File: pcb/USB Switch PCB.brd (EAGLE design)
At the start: 26.7 x 77.5 mm, 28 parts, among them Q1 2N7002P, Q2 2N7002P, U1 D1MINI, X1 AMPHENOL-0001LF, X2 UE27-USBA

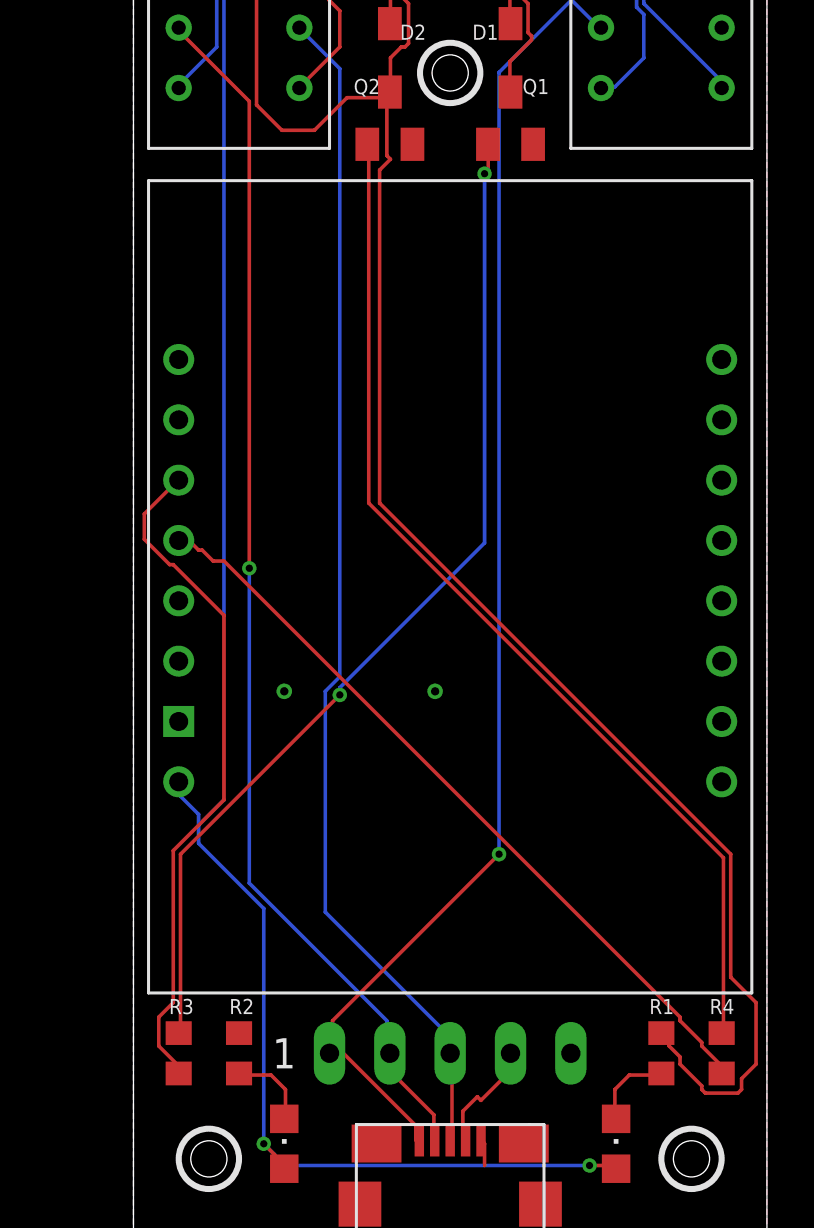
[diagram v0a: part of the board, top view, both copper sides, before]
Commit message: Working on new board revision.
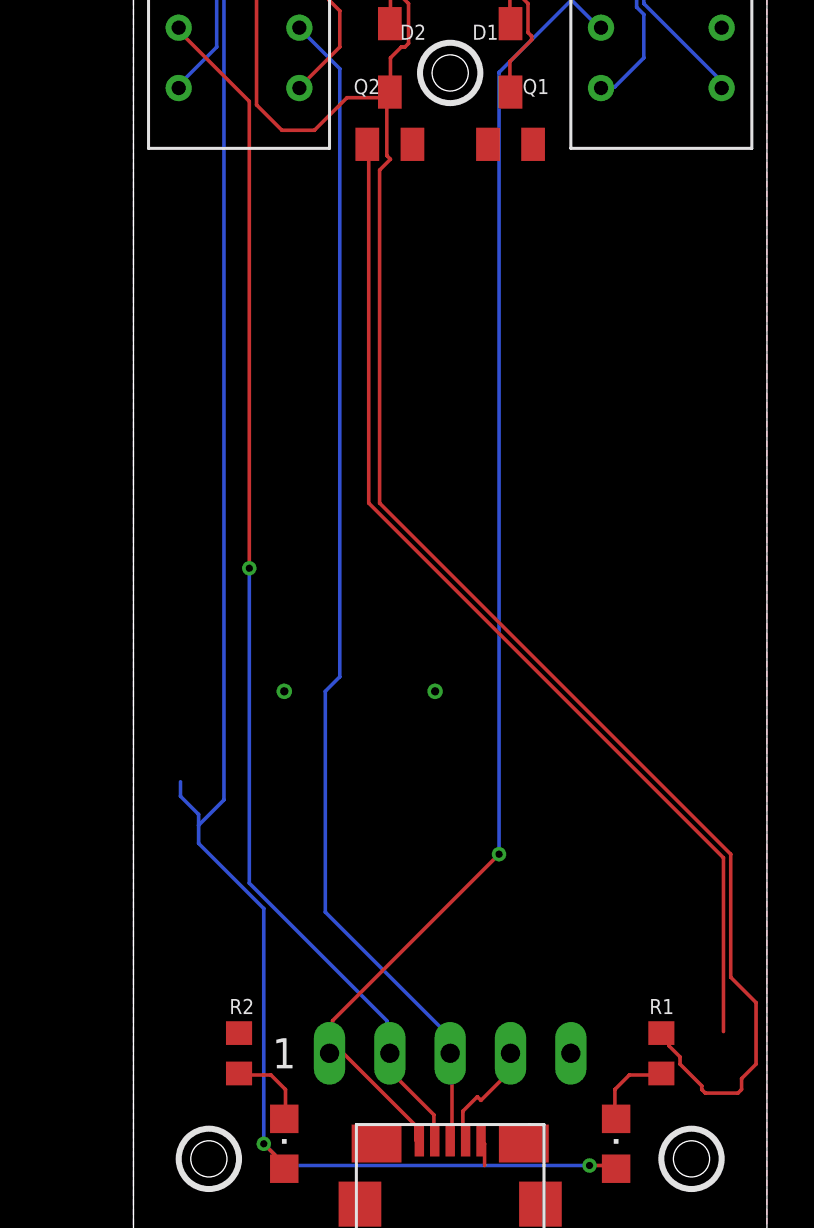
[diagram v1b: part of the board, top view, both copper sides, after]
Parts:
- removed R3, R4: 1kΩ, rcl:R0603
- removed U1: D1MINI, USB Switch PCB:D1MINI
- R1: value 330Ω -> 1kΩ
- R2: value 330 Ω -> 1kΩ
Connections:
- removed net DATAON: MCU.13, R4.1, U1.D2
- removed net N$3: Q1.1, R3.2
- removed net N$4: Q2.1, R4.2
- removed net PWRON: MCU.14, R3.1, U1.D1
- new net DATAGATE: MCU.14, Q2.1
- new net POWERGATE: MCU.13, Q1.1
- net +5V: no longer U1.5V
- net GND: no longer U1.GND
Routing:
- net N$4: track 43.7 -> 0.00 mm
- net DATAGATE: track 0.00 -> 43.6 mm
- net N$3: track 42.8 -> 0.00 mm, vias 2 -> 0
- net DATAON: track 32.5 -> 0.00 mm
- net PWRON: track 28.5 -> 0.00 mm
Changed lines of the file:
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@@
 <attribute name="NAME" x="9.271" y="48.006" size="0.635" layer="25" font="vector"/>
 </element>
-<element name="R1" library="rcl" library_urn="urn:adsk.eagle:library:334" package="R0603" value="330Ω" x="22.225" y="7.62" smashed="yes" rot="R270">
+<element name="R1" library="rcl" library_urn="urn:adsk.eagle:library:334" package="R0603" value="1kΩ" x="22.225" y="7.62" smashed="yes" rot="R270">
 <attribute name="NAME" x="21.717" y="9.271" size="0.635" layer="25" font="vector"/>
 </element>
-<element name="R2" library="rcl" library_urn="urn:adsk.eagle:library:334" package="R0603" value="330 Ω" x="4.445" y="7.62" smashed="yes" rot="R90">
+<element name="R2" library="rcl" library_urn="urn:adsk.eagle:library:334" package="R0603" value="1kΩ" x="4.445" y="7.62" smashed="yes" rot="R90">
 <attribute name="NAME" x="5.08" y="9.906" size="0.635" layer="25" font="vector" rot="R180"/>
-</element>
-<element name="R3" library="rcl" library_urn="urn:adsk.eagle:library:334" package="R0603" value="1kΩ" x="1.905" y="7.62" smashed="yes" rot="R90">
-<attribute name="NAME" x="2.54" y="9.906" size="0.635" layer="25" font="vector" rot="R180"/>
-</element>
-<element name="R4" library="rcl" library_urn="urn:adsk.eagle:library:334" package="R0603" value="1kΩ" x="24.765" y="7.62" smashed="yes" rot="R90">
-<attribute name="NAME" x="24.257" y="9.271" size="0.635" layer="25" font="vector"/>
 </element>
 <element name="S1" library="USB Switch PCB" package="SWITCH" value="SWITCH" x="15.875" y="57.15" smashed="yes" rot="R180"/>
 <element name="U$1" library="USB Switch PCB" package="EC2-5NU" value="EC2-5NUEC2-5NU" x="22.225" y="55.88" smashed="yes" rot="R180"/>
 <element name="U$2" library="USB Switch PCB" package="EC2-5NU" value="EC2-5NUEC2-5NU" x="4.445" y="55.88" smashed="yes" rot="R180"/>
-<element name="U1" library="USB Switch PCB" package="D1MINI" value="D1MINI" x="1.905" y="19.05" smashed="yes"/>
 <element name="UIN" library="USB Switch PCB" package="FE05-1" value="" x="13.335" y="7.62" smashed="yes">
 <attribute name="MF" value="" x="13.335" y="7.62" size="1.778" layer="27" display="off"/>
@@
 <contactref element="Q2" pad="2"/>
 <contactref element="R2" pad="2"/>
-<contactref element="U1" pad="GND"/>
 <contactref element="X1" pad="GND"/>
 <contactref element="UIN" pad="5"/>
@@
 <wire x1="12.7" y1="22.86" x2="11.745" y2="45.89" width="0" layer="19" extent="1-1"/>
 <wire x1="6.35" y1="22.86" x2="12.7" y2="22.86" width="0" layer="19" extent="1-1"/>
-<wire x1="1.905" y1="21.59" x2="6.35" y2="22.86" width="0" layer="19" extent="1-1"/>
-<wire x1="4.445" y1="8.47" x2="1.905" y2="21.59" width="0" layer="19" extent="1-1"/>
+<wire x1="4.445" y1="8.47" x2="6.35" y2="22.86" width="0" layer="19" extent="1-1"/>
 <wire x1="10.235" y1="3.82" x2="4.445" y2="8.47" width="0" layer="19" extent="1-1"/>
 <wire x1="9.535" y1="1.27" x2="10.235" y2="3.82" width="0" layer="19" extent="1-1"/>
@@
 <contactref element="D1" pad="3"/>
 <contactref element="S1" pad="S"/>
-<contactref element="U1" pad="5V"/>
 <contactref element="EXTPWR" pad="1"/>
 <wire x1="21.0312" y1="59.7408" x2="19.812" y2="58.5216" width="0.1524" layer="1"/>
@@
 <wire x1="1.9812" y1="19.05" x2="1.9812" y2="18.4404" width="0.1524" layer="16"/>
 <wire x1="6.2484" y1="2.8956" x2="6.35" y2="2.76" width="0.1524" layer="1"/>
-<wire x1="1.9812" y1="19.05" x2="1.905" y2="19.05" width="0.1524" layer="16"/>
 <wire x1="19.2024" y1="2.8956" x2="20.2692" y2="2.8956" width="0.1524" layer="1"/>
 <wire x1="6.4008" y1="2.8956" x2="19.2024" y2="2.8956" width="0.1524" layer="16"/>
@@
 <wire x1="16.9164" y1="53.0352" x2="16.825" y2="53.17" width="0.1524" layer="1"/>
 </signal>
-<signal name="PWRON">
-<contactref element="U1" pad="D1"/>
-<contactref element="R3" pad="1"/>
-<wire x1="1.8288" y1="7.1628" x2="1.8288" y2="6.858" width="0.1524" layer="1"/>
-<wire x1="1.0668" y1="7.9248" x2="1.8288" y2="7.1628" width="0.1524" layer="1"/>
-<wire x1="1.0668" y1="9.144" x2="1.0668" y2="7.9248" width="0.1524" layer="1"/>
-<wire x1="1.6764" y1="9.7536" x2="1.0668" y2="9.144" width="0.1524" layer="1"/>
-<wire x1="1.6764" y1="16.1544" x2="1.6764" y2="9.7536" width="0.1524" layer="1"/>
-<wire x1="3.81" y1="18.288" x2="1.6764" y2="16.1544" width="0.1524" layer="1"/>
-<wire x1="3.81" y1="26.0604" x2="3.81" y2="18.288" width="0.1524" layer="1"/>
-<wire x1="1.6764" y1="28.194" x2="3.81" y2="26.0604" width="0.1524" layer="1"/>
-<wire x1="1.524" y1="28.194" x2="1.6764" y2="28.194" width="0.1524" layer="1"/>
-<wire x1="0.4572" y1="29.2608" x2="1.524" y2="28.194" width="0.1524" layer="1"/>
-<wire x1="0.4572" y1="30.3276" x2="0.4572" y2="29.2608" width="0.1524" layer="1"/>
-<wire x1="1.8288" y1="31.6992" x2="0.4572" y2="30.3276" width="0.1524" layer="1"/>
-<wire x1="1.8288" y1="6.858" x2="1.905" y2="6.77" width="0.1524" layer="1"/>
-<wire x1="1.8288" y1="31.6992" x2="1.905" y2="31.75" width="0.1524" layer="1"/>
-<contactref element="MCU" pad="14"/>
-<wire x1="-13.645" y1="10.095" x2="1.0668" y2="9.144" width="0" layer="19" extent="1-1"/>
-</signal>
-<signal name="N$3">
-<contactref element="Q1" pad="1"/>
-<contactref element="R3" pad="2"/>
-<wire x1="1.9812" y1="16.002" x2="1.9812" y2="8.5344" width="0.1524" layer="1"/>
-<wire x1="8.6868" y1="22.7076" x2="1.9812" y2="16.002" width="0.1524" layer="1"/>
-<wire x1="8.6868" y1="23.0124" x2="8.6868" y2="22.7076" width="0.1524" layer="16"/>
-<wire x1="14.7828" y1="29.1084" x2="8.6868" y2="23.0124" width="0.1524" layer="16"/>
-<wire x1="14.7828" y1="44.6532" x2="14.7828" y2="29.1084" width="0.1524" layer="16"/>
-<wire x1="14.9352" y1="44.8056" x2="14.7828" y2="44.6532" width="0.1524" layer="1"/>
-<wire x1="14.9352" y1="45.8724" x2="14.9352" y2="44.8056" width="0.1524" layer="1"/>
-<wire x1="1.9812" y1="8.5344" x2="1.905" y2="8.47" width="0.1524" layer="1"/>
-<wire x1="14.9352" y1="45.8724" x2="14.925" y2="45.89" width="0.1524" layer="1"/>
-<via x="8.6868" y="22.7076" extent="1-16" drill="0.3048"/>
-<via x="14.7828" y="44.6532" extent="1-16" drill="0.3048"/>
-</signal>
-<signal name="N$4">
-<contactref element="R4" pad="2"/>
+<signal name="DATAGATE">
 <contactref element="Q2" pad="1"/>
 <wire x1="24.8412" y1="15.8496" x2="24.8412" y2="8.5344" width="0.1524" layer="1"/>
 <wire x1="9.906" y1="30.7848" x2="24.8412" y2="15.8496" width="0.1524" layer="1"/>
 <wire x1="9.906" y1="45.8724" x2="9.906" y2="30.7848" width="0.1524" layer="1"/>
-<wire x1="24.8412" y1="8.5344" x2="24.765" y2="8.47" width="0.1524" layer="1"/>
 <wire x1="9.906" y1="45.8724" x2="9.845" y2="45.89" width="0.1524" layer="1"/>
+<contactref element="MCU" pad="14"/>
+<wire x1="-13.645" y1="10.095" x2="9.906" y2="30.7848" width="0" layer="19" extent="1-1"/>
 </signal>
 <signal name="VCC0">
@@
 <wire x1="13.8684" y1="3.9624" x2="13.985" y2="3.95" width="0.1524" layer="1"/>
 <wire x1="15.8496" y1="7.62" x2="15.875" y2="7.62" width="0.1524" layer="1"/>
-</signal>
-<signal name="DATAON">
-<contactref element="U1" pad="D2"/>
-<contactref element="R4" pad="1"/>
-<wire x1="24.6888" y1="7.1628" x2="24.6888" y2="6.858" width="0.1524" layer="1"/>
-<wire x1="23.9268" y1="7.9248" x2="24.6888" y2="7.1628" width="0.1524" layer="1"/>
-<wire x1="23.9268" y1="8.0772" x2="23.9268" y2="7.9248" width="0.1524" layer="1"/>
-<wire x1="23.0124" y1="8.9916" x2="23.9268" y2="8.0772" width="0.1524" layer="1"/>
-<wire x1="23.0124" y1="9.144" x2="23.0124" y2="8.9916" width="0.1524" layer="1"/>
-<wire x1="3.81" y1="28.3464" x2="23.0124" y2="9.144" width="0.1524" layer="1"/>
-<wire x1="3.3528" y1="28.3464" x2="3.81" y2="28.3464" width="0.1524" layer="1"/>
-<wire x1="2.8956" y1="28.8036" x2="3.3528" y2="28.3464" width="0.1524" layer="1"/>
-<wire x1="2.7432" y1="28.8036" x2="2.8956" y2="28.8036" width="0.1524" layer="1"/>
-<wire x1="2.4384" y1="29.1084" x2="2.7432" y2="28.8036" width="0.1524" layer="1"/>
-<wire x1="1.9812" y1="29.1084" x2="2.4384" y2="29.1084" width="0.1524" layer="1"/>
-<wire x1="24.6888" y1="6.858" x2="24.765" y2="6.77" width="0.1524" layer="1"/>
-<wire x1="1.9812" y1="29.1084" x2="1.905" y2="29.21" width="0.1524" layer="1"/>
-<contactref element="MCU" pad="13"/>
-<wire x1="-13.645" y1="8.095" x2="1.9812" y2="29.1084" width="0" layer="19" extent="1-1"/>
 </signal>
 <signal name="N$5">
@@
 <wire x1="-25.4" y1="-14.125" x2="-20.955" y2="-52.705" width="0" layer="19" extent="1-1"/>
 </signal>
+<signal name="POWERGATE">
+<contactref element="Q1" pad="1"/>
+<contactref element="MCU" pad="13"/>
+<wire x1="-13.645" y1="8.095" x2="14.925" y2="45.89" width="0" layer="19" extent="1-1"/>
+</signal>
 </signals>
